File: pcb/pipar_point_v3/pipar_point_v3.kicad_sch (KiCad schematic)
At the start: 21 parts, among them SW3 SW_SPDT, SW5 SW_SPDT

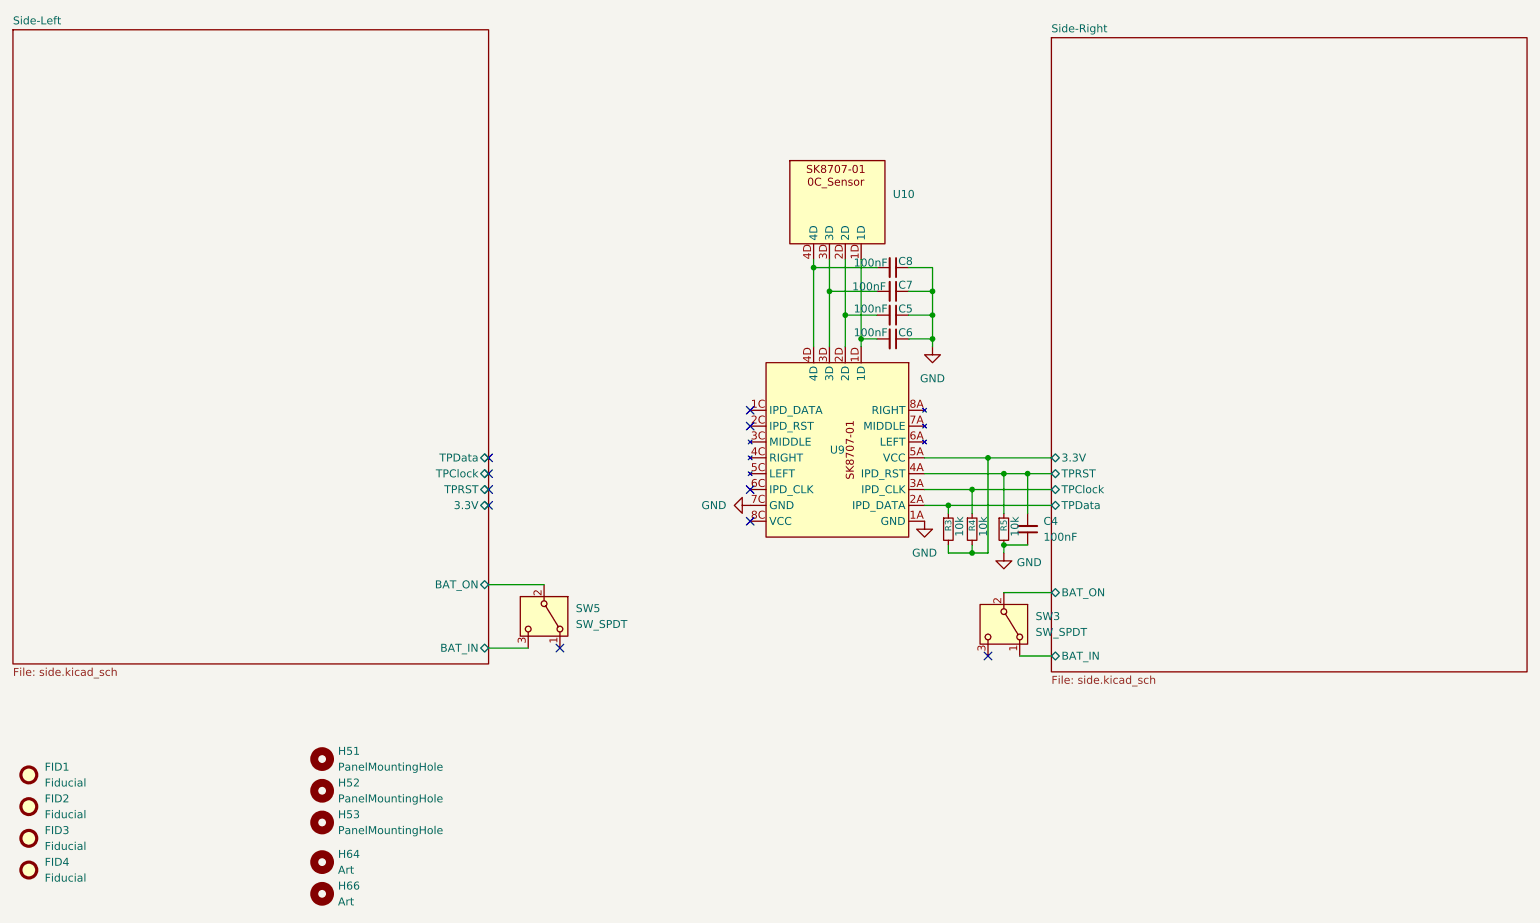
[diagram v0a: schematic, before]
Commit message: do some work for the dongle
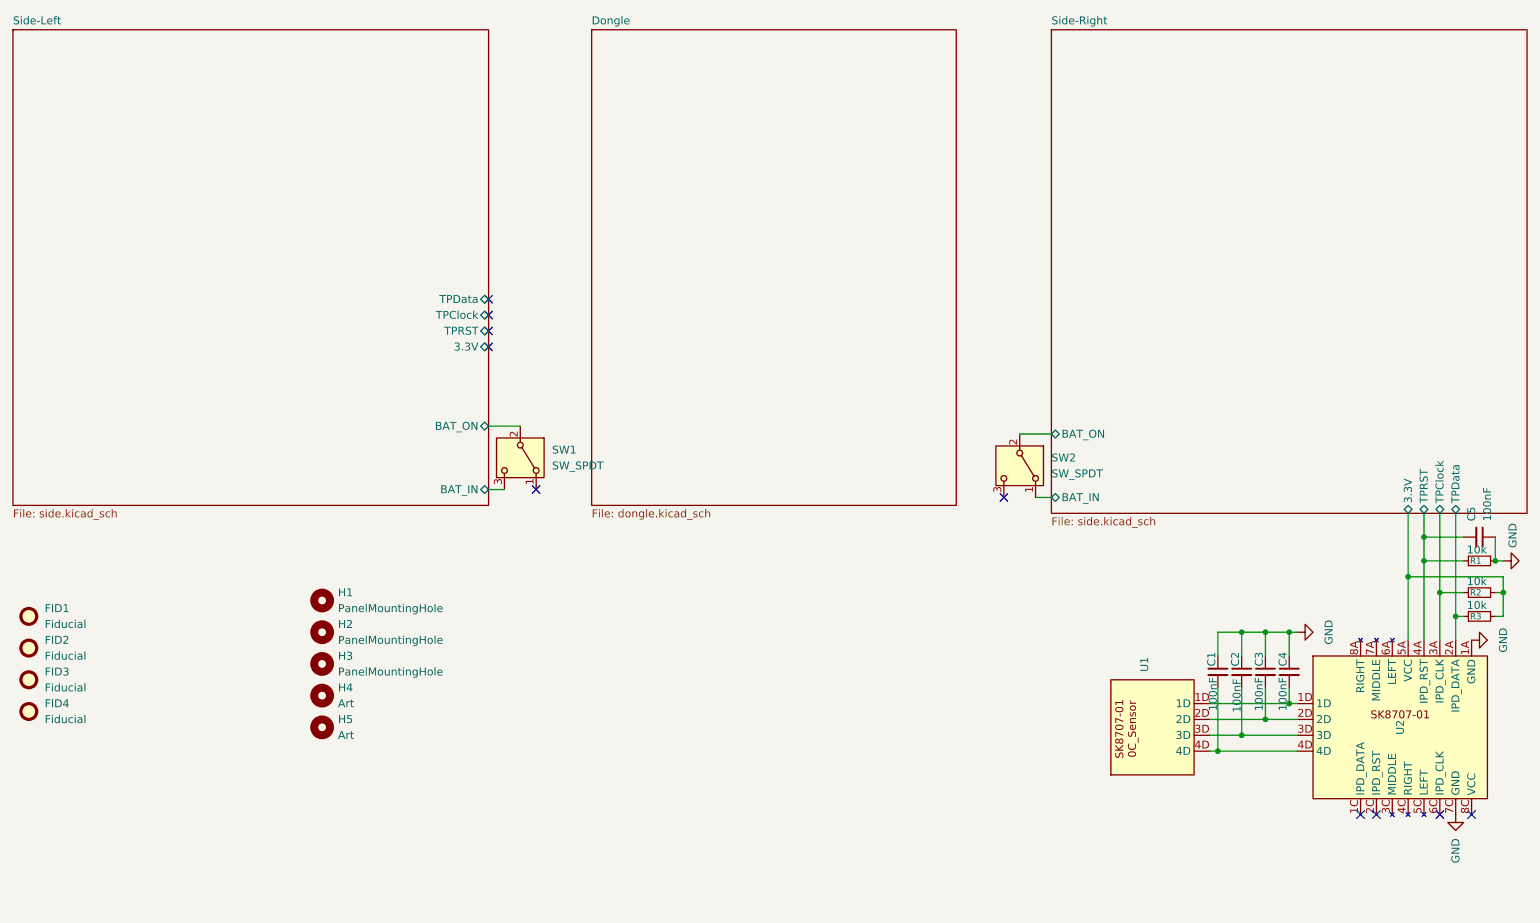
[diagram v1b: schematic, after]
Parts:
- renumbered C8 to C1, C7 to C2, C5 to C3, C6 to C4, C4 to C5, H51 to H1, H52 to H2, H53 to H3, H64 to H4, H66 to H5, R5 to R1, R4 to R2, SW5 to SW1, SW3 to SW2, U10 to U1, U9 to U2
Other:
- added sheet Dongle (dongle.kicad_sch)
- moved on the sheet: C1, C2, C3, C4, C5, FID1, FID2, FID3, FID4, H1, H2, H3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
